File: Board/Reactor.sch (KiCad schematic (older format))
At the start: 20 parts, among them P1 CONN_02X13, P2 USER_PORT, P3 CONN_01X13, P4 LA_PWR, P5 USB_OTG, P6 DEBUG, U1 usb1232h, U2 PCF8574

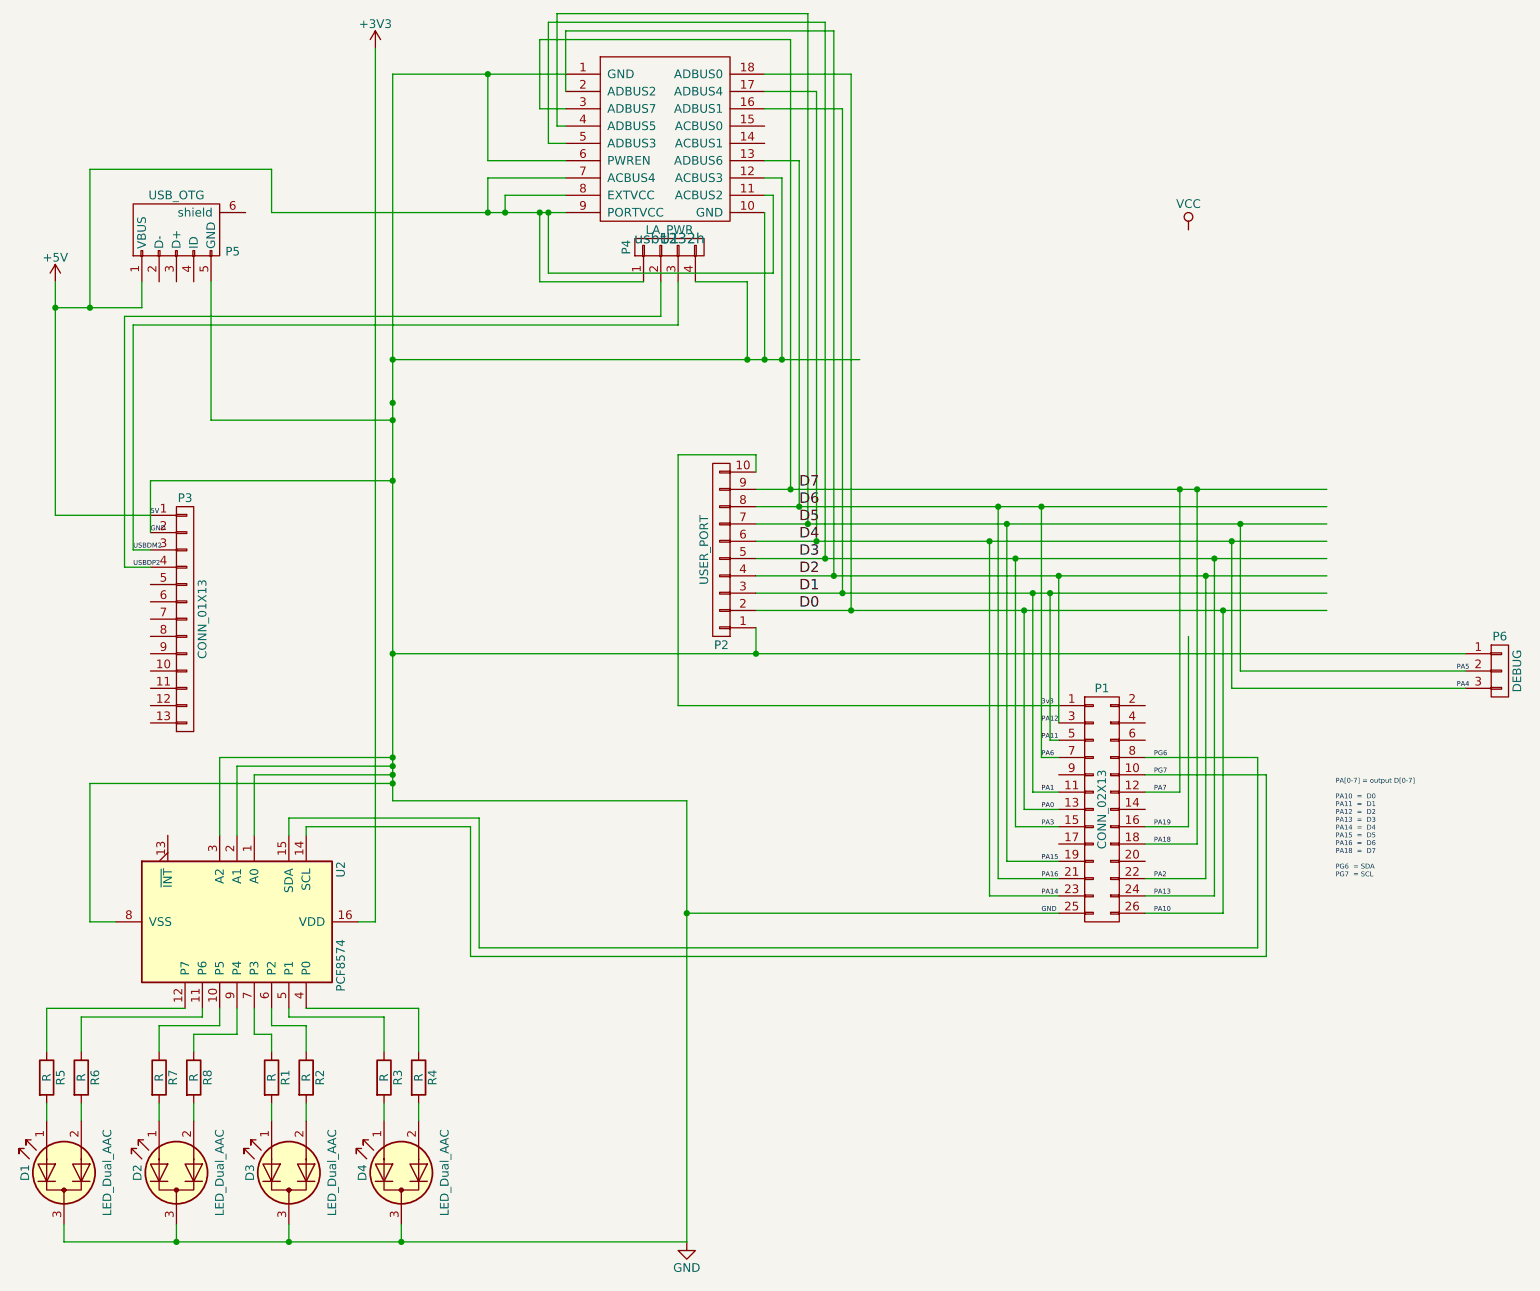
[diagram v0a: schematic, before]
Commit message: - board laid out (draft).
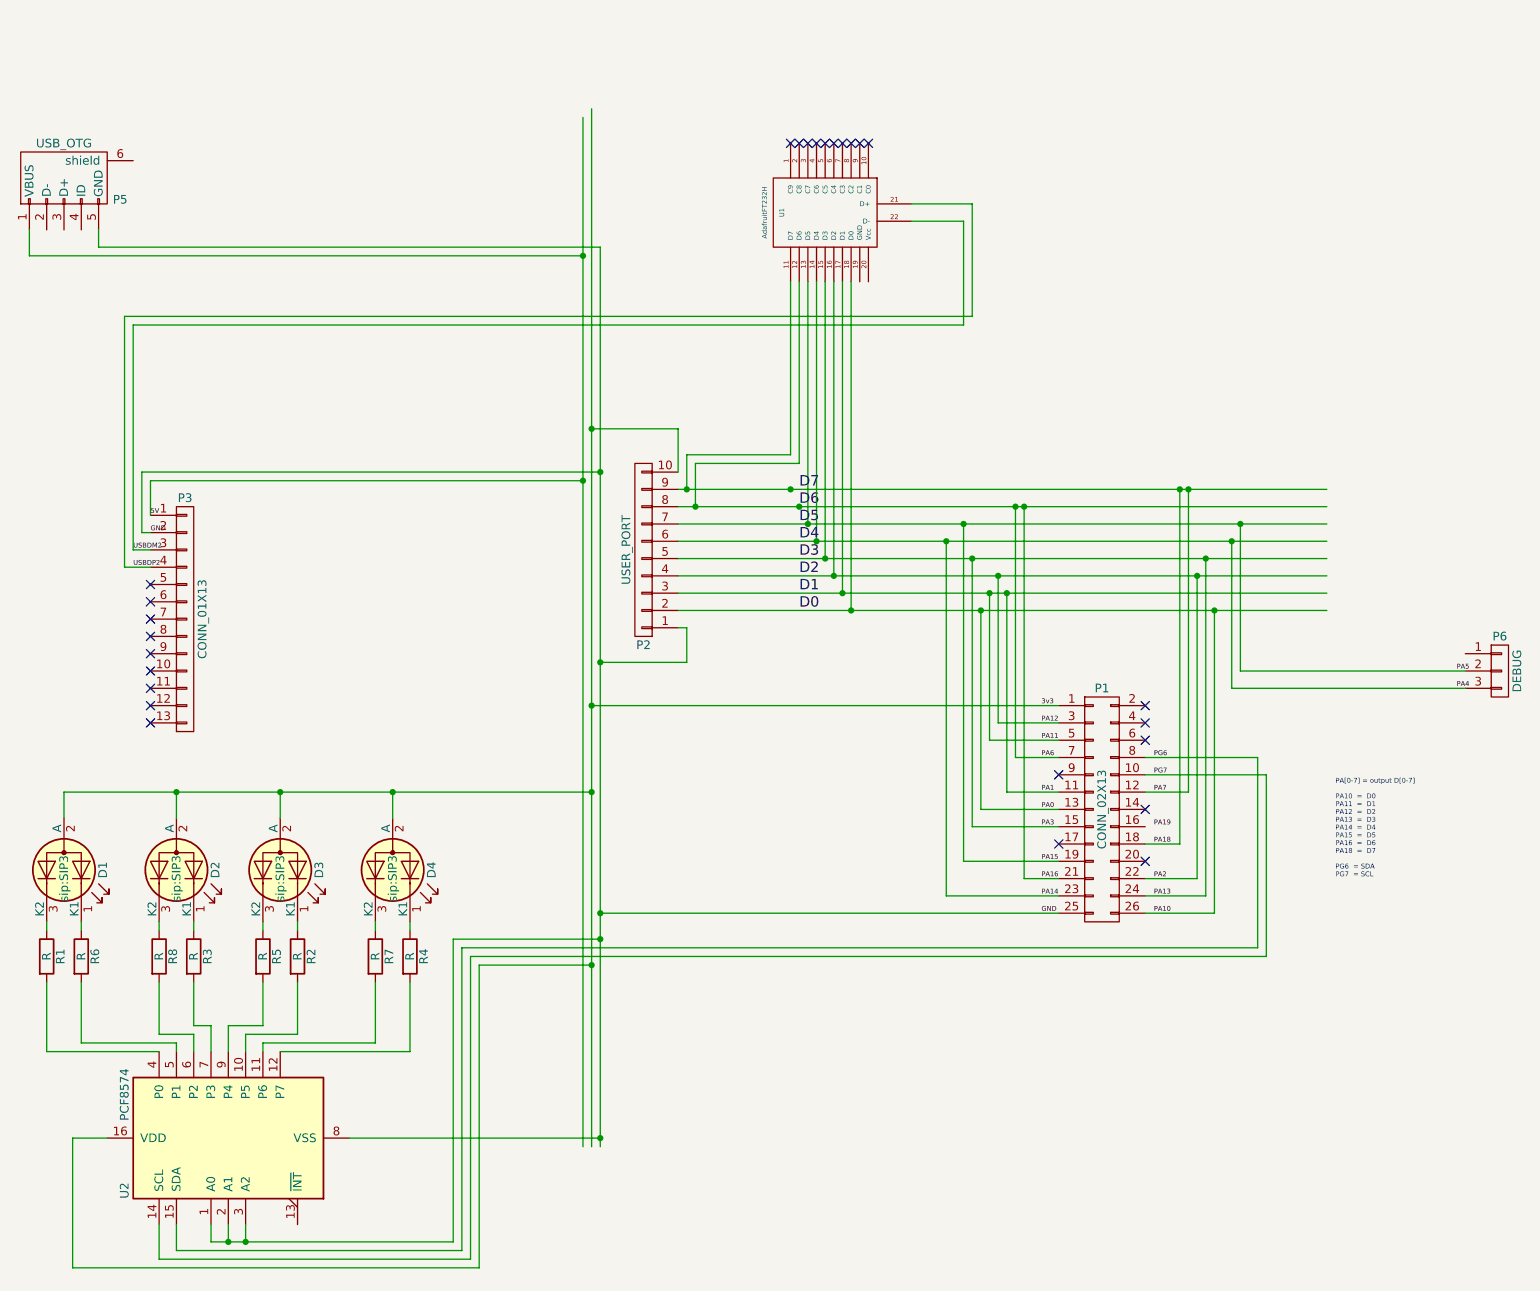
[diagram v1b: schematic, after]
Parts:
- removed D1, D2, D3, D4: LED_Dual_AAC, LEDs_new:LED_D3.0mm-3, symbol LED_Dual_AAC
- removed P4: LA_PWR, Connectors_Molex:Molex_KK-6410-04_04x2.54mm_Straight, symbol CONN_01X04
- removed U1: usb1232h, Housings_DIP:DIP-18_W7.62mm_LongPads, symbol usb1232h
- added D1, D2, D3, D4: LED_Dual_CAC, sip:SIP3, symbol LED_Dual_CAC
- added U1: AdafruitFT232H, ReactorProject:AdafruitFT232h, symbol AdafruitFT232H
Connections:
- net labels removed: +3V3, +5V, VCC
- wire segments 171 -> 140
- no-connect marks 0 -> 26
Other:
- moved on the sheet: P2, P5, R2, R4, R6, R8, U2

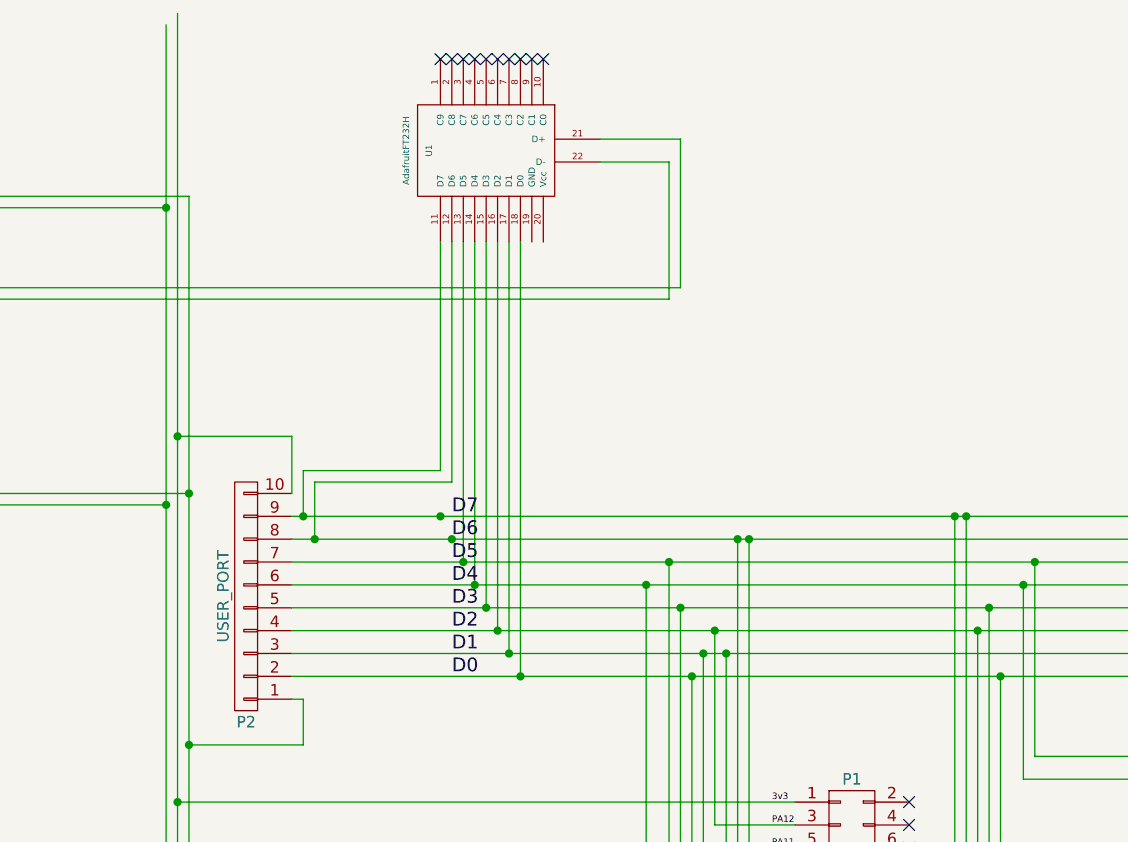
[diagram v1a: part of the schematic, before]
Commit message: - Getting PCB ready for manufacture
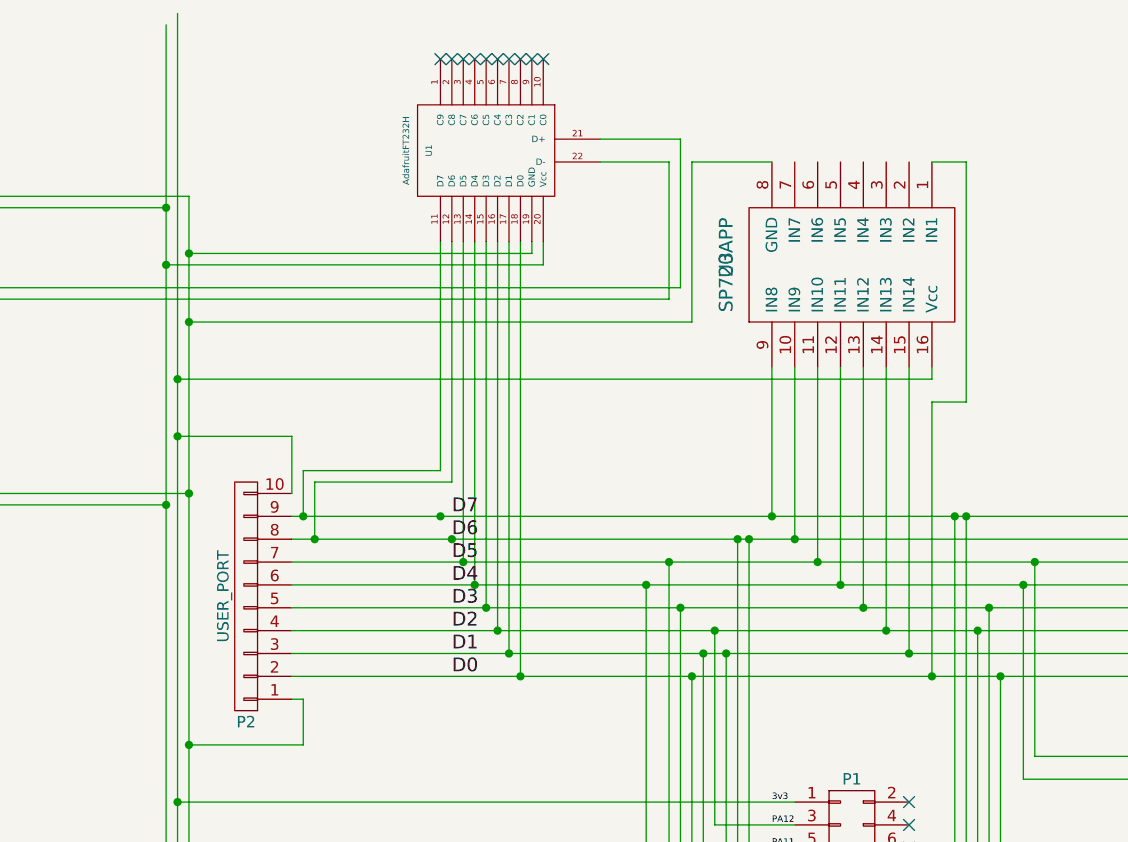
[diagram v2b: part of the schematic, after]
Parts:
- added U3: SP720APP, dip:DIP16, symbol SP720APP
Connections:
- wire segments 140 -> 160
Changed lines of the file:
@@
 Text Label 7750 4750 0    28   ~ 0
 PA11
+$Comp
+L SP720APP U3
+U 1 1 59026405
+P 7550 2200
+F 0 "U3" H 7550 2200 60  0000 C CNN
+F 1 "SP720APP" H 7550 2200 60  0000 C CNN
+F 2 "dip:DIP16" H 7550 2200 60  0001 C CNN
+F 3 "" H 7550 2200 60  0001 C CNN
+	1    7550 2200
+	0    1    1    0
+$EndComp
 Wire Wire Line
 	5650 4000 9400 4000
@@
 	5700 4300 5200 4300
 Connection ~ 5200 4300
+Wire Wire Line
+	7750 2650 7750 3300
+Connection ~ 7750 3300
+Wire Wire Line
+	7850 2650 7850 3400
+Connection ~ 7850 3400
+Wire Wire Line
+	7950 2650 7950 3500
+Connection ~ 7950 3500
+Wire Wire Line
+	8050 2650 8050 3600
+Connection ~ 8050 3600
+Wire Wire Line
+	8150 2650 8150 3700
+Connection ~ 8150 3700
+Wire Wire Line
+	8250 2650 8250 3800
+Connection ~ 8250 3800
+Wire Wire Line
+	8350 2650 8350 3900
+Connection ~ 8350 3900
+Wire Wire Line
+	8450 1750 8600 1750
+Wire Wire Line
+	8600 1750 8600 2800
+Wire Wire Line
+	8600 2800 8450 2800
+Wire Wire Line
+	8450 2800 8450 4000
+Connection ~ 8450 4000
+Wire Wire Line
+	7750 1750 7400 1750
+Wire Wire Line
+	7400 1750 7400 2450
+Wire Wire Line
+	7400 2450 5200 2450
+Connection ~ 5200 2450
+Wire Wire Line
+	8450 2650 8450 2700
+Wire Wire Line
+	8450 2700 5150 2700
+Connection ~ 5150 2700
+Wire Wire Line
+	6700 2100 6700 2150
+Wire Wire Line
+	6700 2150 5200 2150
+Connection ~ 5200 2150
+Wire Wire Line
+	6750 2100 6750 2200
+Wire Wire Line
+	6750 2200 5100 2200
+Connection ~ 5100 2200
 $EndSCHEMATC
